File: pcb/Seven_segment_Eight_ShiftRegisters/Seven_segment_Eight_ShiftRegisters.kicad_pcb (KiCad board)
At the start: 2 copper layers, 68 parts, among them J1 B5B-XH-A_LF__SN_, J2 B3B-PH-K-S_LF__SN_, Q1 TIP120, Q2 TIP120, Q3 TIP120, Q4 TIP120, Q5 TIP120, U1 5161AS, U10 5161AS, U11 5161AS, U12 74HC595, U13 5161AS, U14 5161AS, U15 5161AS, U16 5161AS, U17 5161AS, U18 74HC595, U19 5161AS, U2 5161AS, U20 5161AS, U21 5161AS, U22 5161AS, U23 5161AS, U24 74HC595, U25 5161AS, U26 5161AS, U27 5161AS, U28 5161AS, U29 5161AS, U3 5161AS, U30 74HC595, U31 5161AS, U32 5161AS, U33 5161AS, U34 5161AS, U35 5161AS, U36 74HC595, U37 5161AS, U38 5161AS, U39 5161AS, U4 5161AS, U40 5161AS, U41 5161AS, U42 74HC595, U43 5161AS, U44 5161AS, U45 5161AS, U46 5161AS, U47 5161AS, U48 74HC595, U5 5161AS, U6 74HC595, U7 5161AS, U8 5161AS, U9 5161AS

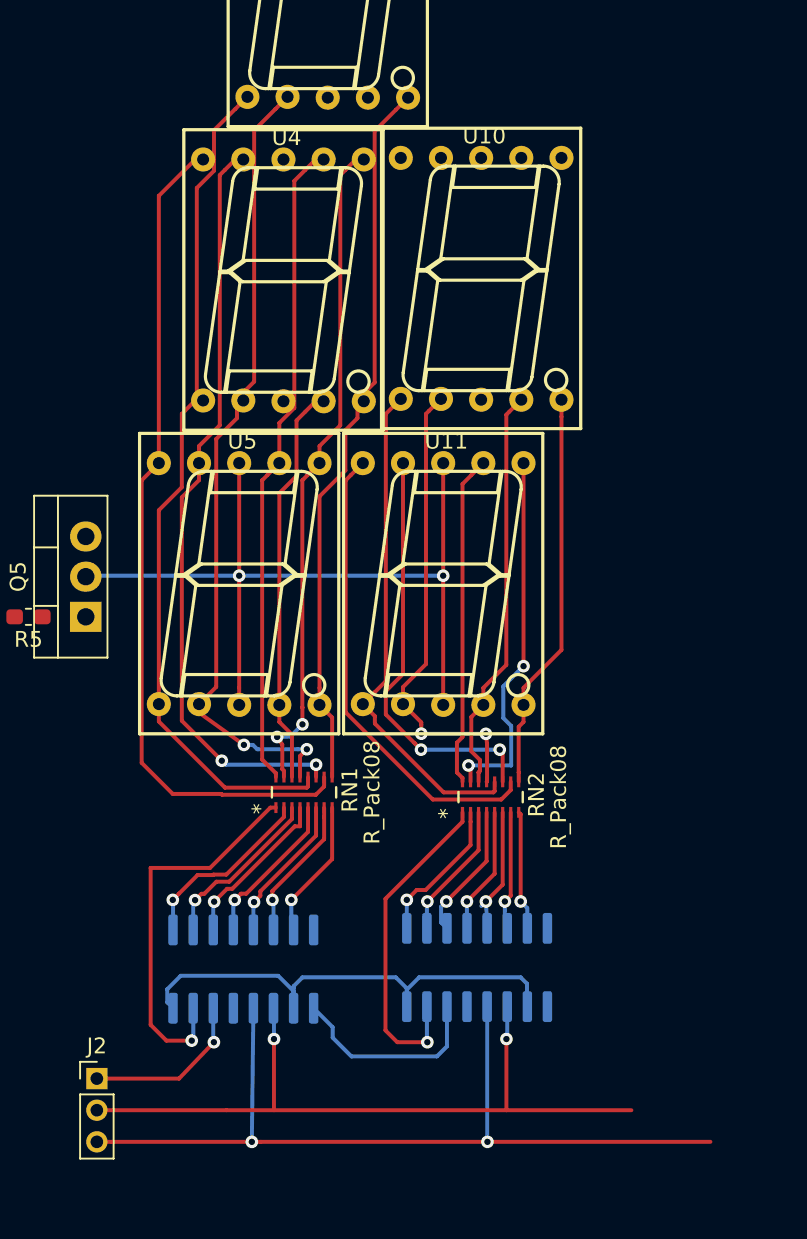
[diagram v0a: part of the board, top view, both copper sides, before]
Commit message: About to duplicate 3d models
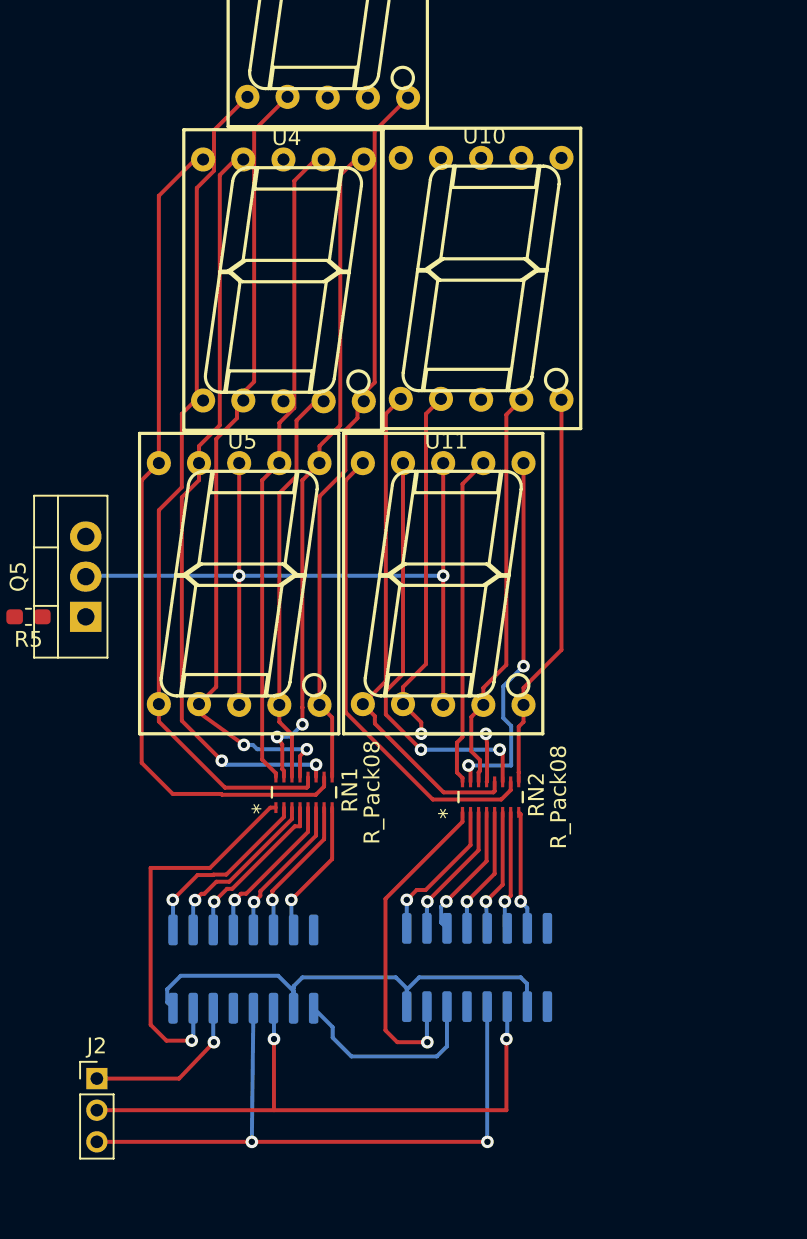
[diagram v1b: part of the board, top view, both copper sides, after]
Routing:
- net Net-(J2-Pad3): track 55.8 -> 41.7 mm
- net Net-(J2-Pad2): track 46.8 -> 38.9 mm
